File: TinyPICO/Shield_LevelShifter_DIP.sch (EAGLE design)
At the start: 10 parts, among them U1 SN74HCT245N

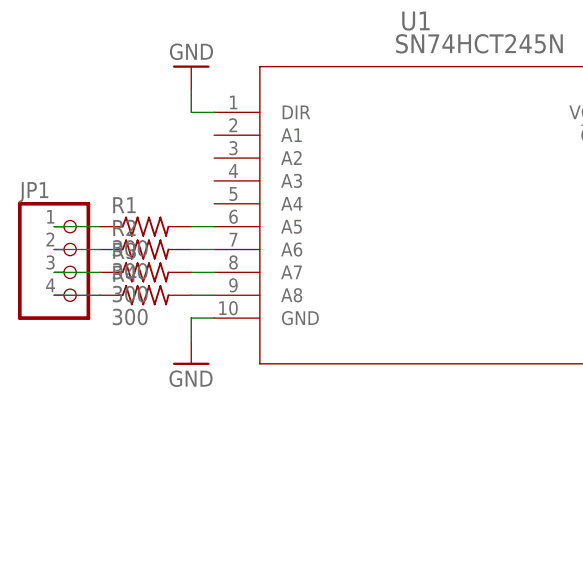
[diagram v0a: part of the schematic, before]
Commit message: Prettier
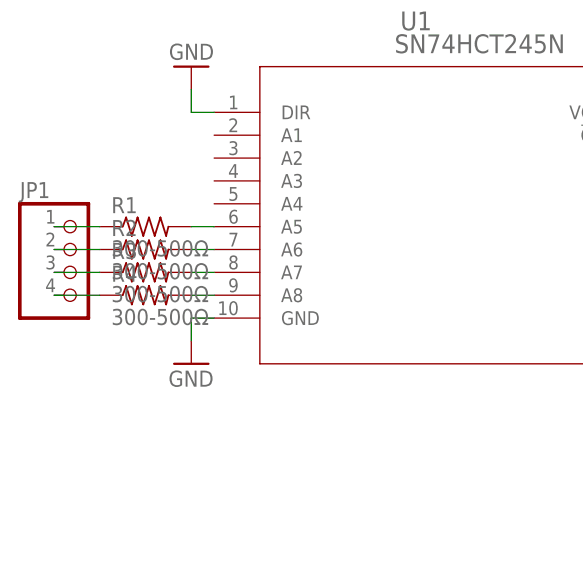
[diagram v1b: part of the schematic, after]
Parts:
- R1, R2, R3, R4: value 300 -> 300-500Ω
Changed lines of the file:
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@@
 <part name="RIGHT" library="UnexpectedMaker" deviceset="TINYPICO_HEADER_10" device="NO_SILK_PTH_FEMALE"/>
 <part name="LOGO1" library="SparkFun-Aesthetics" library_urn="urn:adsk.eagle:library:507" deviceset="OSHW-LOGO" device="S" package3d_urn="urn:adsk.eagle:package:37099/1" value="OSHW-LOGOS"/>
-<part name="R1" library="rcl" library_urn="urn:adsk.eagle:library:334" deviceset="R-US_" device="0204/2V" package3d_urn="urn:adsk.eagle:package:23495/1" value="300"/>
-<part name="R2" library="rcl" library_urn="urn:adsk.eagle:library:334" deviceset="R-US_" device="0204/2V" package3d_urn="urn:adsk.eagle:package:23495/1" value="300"/>
-<part name="R3" library="rcl" library_urn="urn:adsk.eagle:library:334" deviceset="R-US_" device="0204/2V" package3d_urn="urn:adsk.eagle:package:23495/1" value="300"/>
-<part name="R4" library="rcl" library_urn="urn:adsk.eagle:library:334" deviceset="R-US_" device="0204/2V" package3d_urn="urn:adsk.eagle:package:23495/1" value="300"/>
+<part name="R1" library="rcl" library_urn="urn:adsk.eagle:library:334" deviceset="R-US_" device="0204/2V" package3d_urn="urn:adsk.eagle:package:23495/1" value="300-500Ω"/>
+<part name="R2" library="rcl" library_urn="urn:adsk.eagle:library:334" deviceset="R-US_" device="0204/2V" package3d_urn="urn:adsk.eagle:package:23495/1" value="300-500Ω"/>
+<part name="R3" library="rcl" library_urn="urn:adsk.eagle:library:334" deviceset="R-US_" device="0204/2V" package3d_urn="urn:adsk.eagle:package:23495/1" value="300-500Ω"/>
+<part name="R4" library="rcl" library_urn="urn:adsk.eagle:library:334" deviceset="R-US_" device="0204/2V" package3d_urn="urn:adsk.eagle:package:23495/1" value="300-500Ω"/>
 <part name="P+1" library="supply1" library_urn="urn:adsk.eagle:library:371" deviceset="+5V" device=""/>
 <part name="GND1" library="supply1" library_urn="urn:adsk.eagle:library:371" deviceset="GND" device=""/>
